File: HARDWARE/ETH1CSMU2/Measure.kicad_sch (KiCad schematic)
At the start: 34 parts, among them U401 DG444DY+, U402 DG444DY+, U403 DG419DY, U404 DG419DY, U405 OPA140/OPA141, U406 OPA140/OPA141, U407 ADS8681IRUMT, U408 ADS8681IRUMT

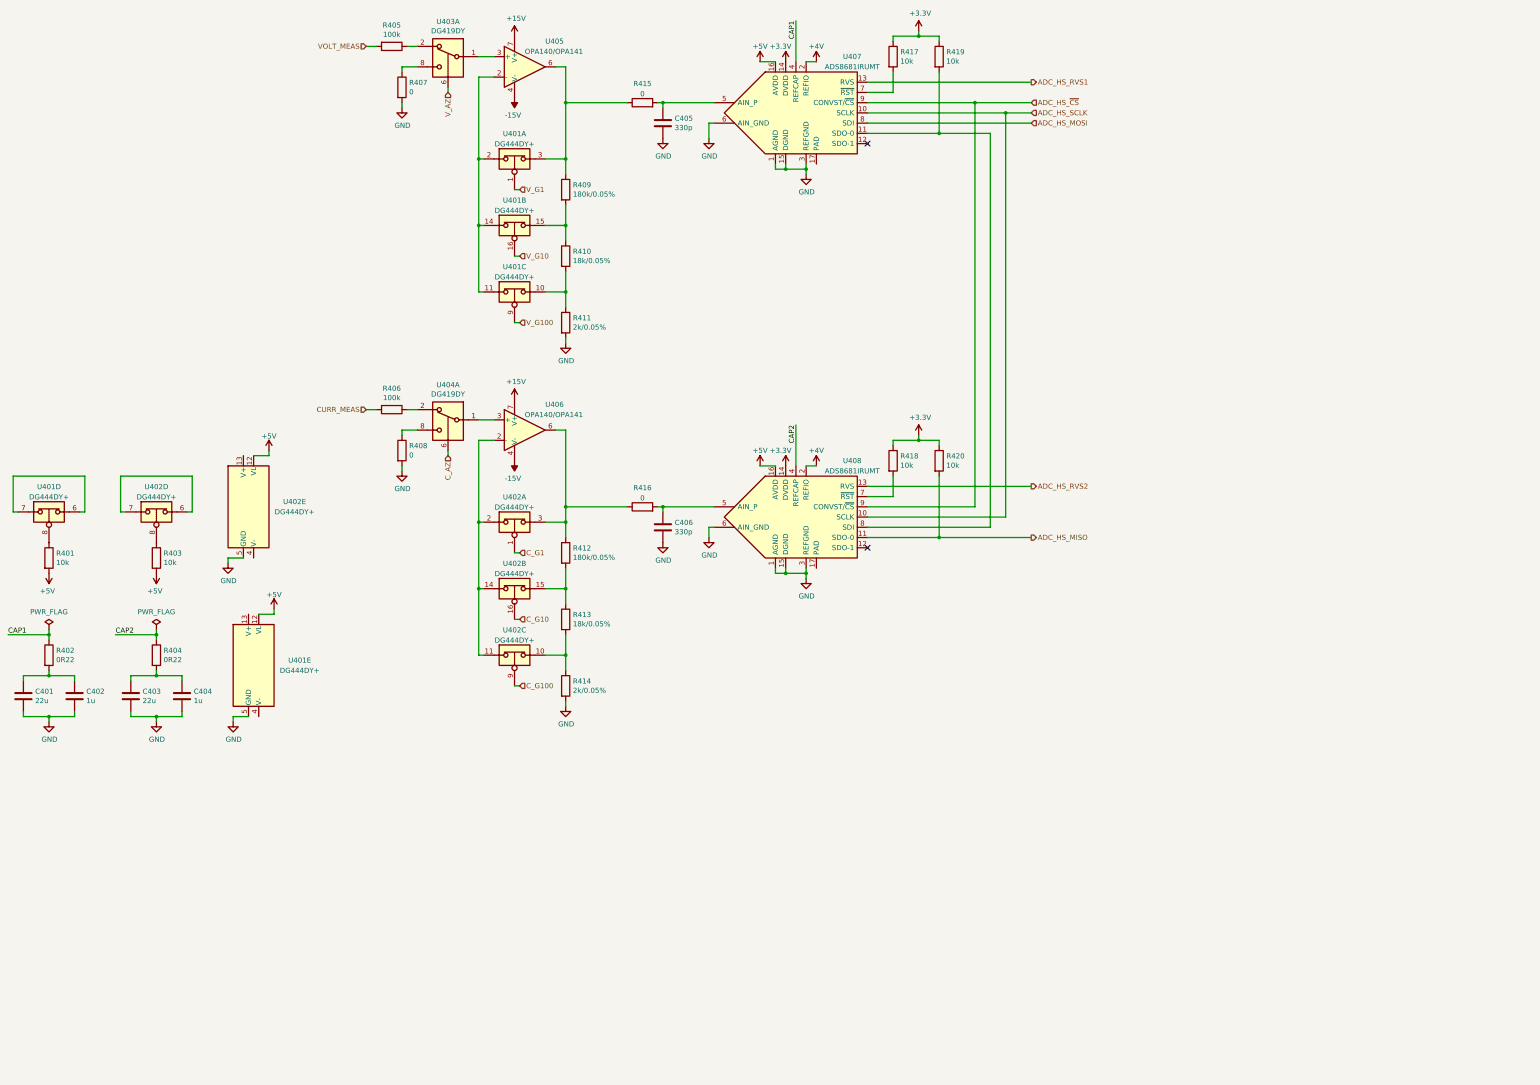
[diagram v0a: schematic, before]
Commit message: Hardware design
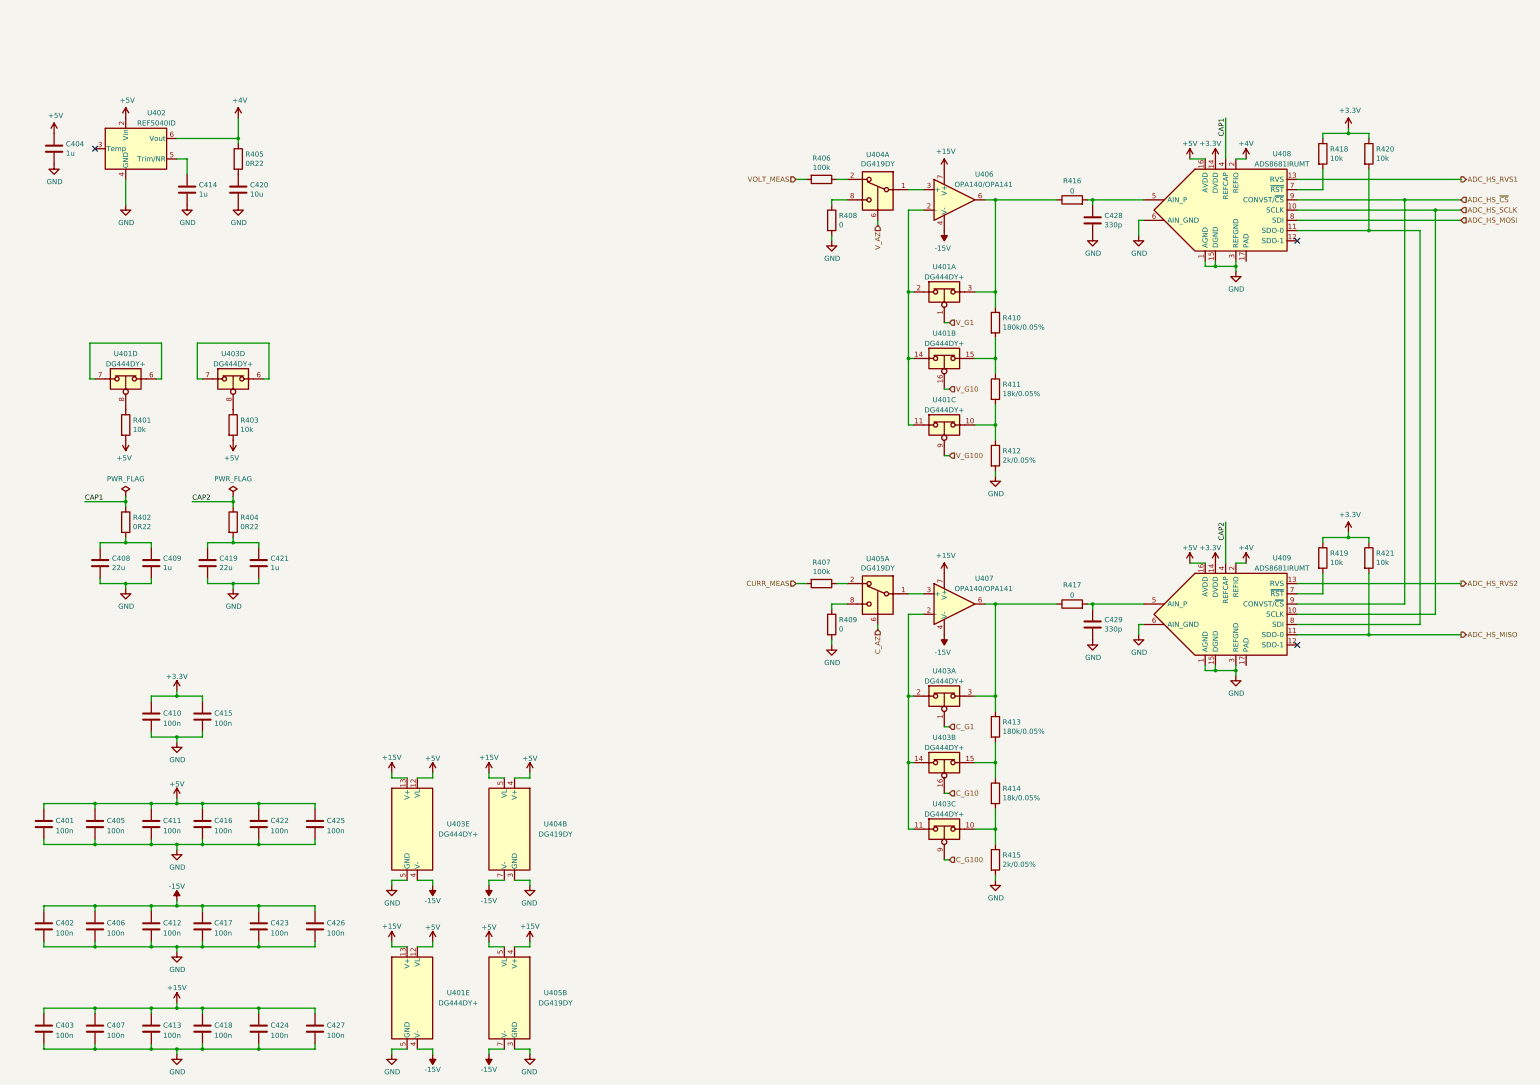
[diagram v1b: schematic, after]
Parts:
- added C401, C402, C403, C405, C406, C407, C410, C411, C412, C413, C415, C416, C417, C418, C422, C423, C424, C425, C426, C427: 100n, symbol Device:C
- added C404, C414: 1u, Capacitor_SMD:C_0603_1608Metric_Pad1.08x0.95mm_HandSolder, symbol Device:C
- added C420: 10u, Resistor_SMD:R_0805_2012Metric_Pad1.20x1.40mm_HandSolder, symbol Device:C
- added R405: 0R22, Resistor_SMD:R_0603_1608Metric_Pad0.98x0.95mm_HandSolder, symbol Device:R
- added U402: REF5040ID, Package_SO:SOIC-8_3.9x4.9mm_P1.27mm, symbol Reference_Voltage:REF5040ID
- added unit 2 of U404
- added unit 2 of U405
- renumbered C401 to C408, C402 to C409, C403 to C419, C404 to C421, C405 to C428, C406 to C429, R405 to R406, R406 to R407, R407 to R408, R408 to R409, R409 to R410, R410 to R411, R411 to R412, R412 to R413, R413 to R414, R414 to R415, R415 to R416, R416 to R417, R417 to R418, R418 to R419, R419 to R420, R420 to R421, U402 to U403, U403 to U404, U404 to U405, U405 to U406, U406 to U407, U407 to U408, U408 to U409
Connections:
- net +15V: now also U401.13 (V+), U403.13 (V+), C403.1, C407.1, C413.1, C418.1, C424.1, C427.1, U404.5 (VL), U405.4 (V+)
- net +3.3V: now also C410.1, C415.1
- net +4V: now also R405.1, U402.6 (Vout)
- net +5V: now also C401.1, C404.1, C405.1, C411.1, C416.1, C422.1, C425.1, U402.2 (Vin), U404.4 (V+), U405.5 (VL)
- net -15V: now also U401.4 (V-), U403.4 (V-), C402.1, C406.1, C412.1, C417.1, C423.1, C426.1, U404.7 (V-), U405.7 (V-)
- net GND: now also C401.2, C402.2, C403.2, C404.2, C405.2, C406.2, C407.2, C410.2, C411.2, C412.2, C413.2, C414.2, C415.2, C416.2, C417.2, C418.2, C420.2, C422.2, C423.2, C424.2, C425.2, C426.2, C427.2, U402.4 (GND), U404.3 (GND), U405.3 (GND)
- new net: C420.1, R405.2
- new net: C414.1, U402.5 (Trim/NR)
- no-connect marks 2 -> 3
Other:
- moved on the sheet: C408, C409, C419, C421, C428, C429, R401, R402, R403, R404, R406, R407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
